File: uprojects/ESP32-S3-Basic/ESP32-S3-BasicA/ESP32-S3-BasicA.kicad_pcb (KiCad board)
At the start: 2 copper layers, 5 parts, among them U1 ESP32-S3-WROOM-1x-N8R8

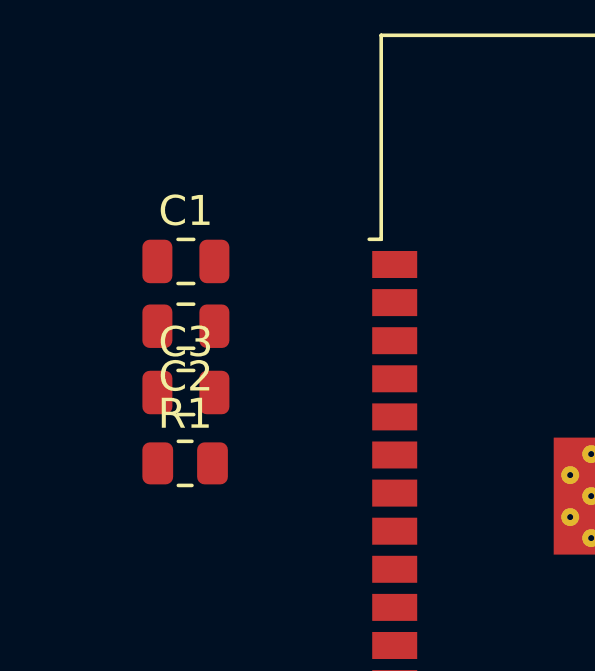
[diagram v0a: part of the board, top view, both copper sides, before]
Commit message: March 27 commit
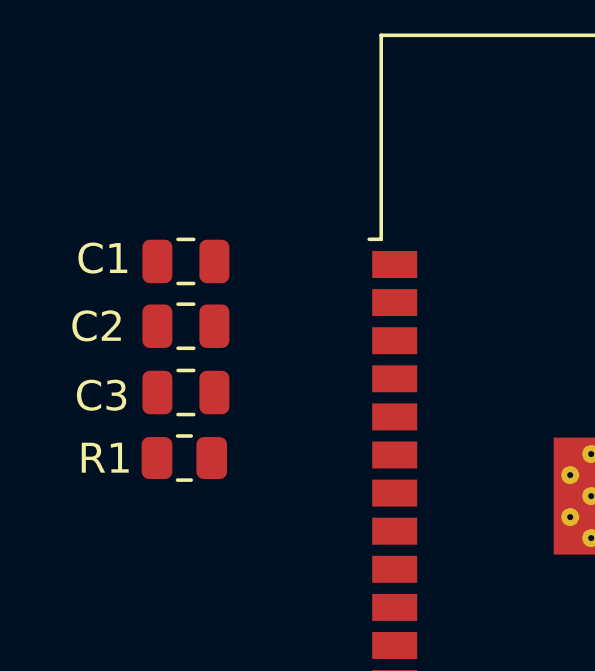
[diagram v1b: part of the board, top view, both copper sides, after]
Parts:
- moved R1 0.18 mm to (134.9, 65.5)
- turned C1 to 180 degrees
- turned C2 to 0 degrees
- turned C3 to 180 degrees
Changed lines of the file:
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@@
   (net 39 "ESP_EN")
   (footprint "Resistor_SMD:R_0805_2012Metric" (layer "F.Cu")
-    (at 134.8994 65.6336)
+    (at 134.874 65.4558)
     (descr "Resistor SMD 0805 (2012 Metric), square (rectangular) end terminal, IPC_7351 nominal, (Body size source: IPC-SM-782 page 72, https://www.pcb-3d.com/wordpress/wp-content/uploads/ipc-sm-782a_amendment_1_and_2.pdf), generated with kicad-footprint-generator")
     (tags "resistor")
@@
     (property "Sheetname" "")
     (attr smd)
-    (fp_text reference "R1" (at 0 -1.65) (layer "F.SilkS")
-        (effects (font (size 1 1) (thickness 0.15)))
-    )
-    (fp_text value "10k/R0402" (at 0 1.65) (layer "F.Fab")
+    (fp_text reference "R1" (at -2.6416 0.0254) (layer "F.SilkS")
+        (effects (font (size 1 1) (thickness 0.15)))
+    )
+    (fp_text value "10k/R0402" (at -7.8994 -8.255) (layer "F.Fab")
         (effects (font (size 1 1) (thickness 0.15)))
     )
@@
   )
   (footprint "Capacitor_SMD:C_0805_2012Metric" (layer "F.Cu")
-    (at 134.9248 61.0616 180)
+    (at 134.9248 61.0616)
     (descr "Capacitor SMD 0805 (2012 Metric), square (rectangular) end terminal, IPC_7351 nominal, (Body size source: IPC-SM-782 page 76, https://www.pcb-3d.com/wordpress/wp-content/uploads/ipc-sm-782a_amendment_1_and_2.pdf, https://docs.google.com/spreadsheets/d/1BsfQQcO9C6DZCsRaXUlFlo91Tg2WpOkGARC1WS5S8t0/edit?usp=sharing), generated with kicad-footprint-generator")
     (tags "capacitor")
@@
     (property "Sheetname" "")
     (attr smd)
-    (fp_text reference "C2" (at 0 -1.68 180) (layer "F.SilkS")
-        (effects (font (size 1 1) (thickness 0.15)))
-    )
-    (fp_text value "100nF/10V/10%/X7R/C0402" (at 6.1214 2.3368 180) (layer "F.Fab")
-        (effects (font (size 1 1) (thickness 0.15)))
-    )
-    (fp_text user "${REFERENCE}" (at 0 0 180) (layer "F.Fab")
+    (fp_text reference "C2" (at -2.9464 0.0254) (layer "F.SilkS")
+        (effects (font (size 1 1) (thickness 0.15)))
+    )
+    (fp_text value "100nF/10V/10%/X7R/C0402" (at -0.889 -7.366) (layer "F.Fab")
+        (effects (font (size 1 1) (thickness 0.15)))
+    )
+    (fp_text user "${REFERENCE}" (at 0 0) (layer "F.Fab")
         (effects (font (size 0.5 0.5) (thickness 0.08)))
     )
@@
     (fp_line (start 1 0.625) (end -1 0.625)
       (stroke (width 0.1) (type solid)) (layer "F.Fab"))
-    (pad "1" smd roundrect (at -0.95 0 180) (size 1 1.45) (layers "F.Cu" "F.Paste" "F.Mask") (roundrect_rratio 0.25)
+    (pad "1" smd roundrect (at -0.95 0) (size 1 1.45) (layers "F.Cu" "F.Paste" "F.Mask") (roundrect_rratio 0.25)
       (net 38 "GND") (pintype "passive"))
-    (pad "2" smd roundrect (at 0.95 0 180) (size 1 1.45) (layers "F.Cu" "F.Paste" "F.Mask") (roundrect_rratio 0.25)
+    (pad "2" smd roundrect (at 0.95 0) (size 1 1.45) (layers "F.Cu" "F.Paste" "F.Mask") (roundrect_rratio 0.25)
       (net 37 "+3.3V") (pintype "passive"))
     (model "${KICAD6_3DMODEL_DIR}/Capacitor_SMD.3dshapes/C_0805_2012Metric.wrl"
@@
   )
   (footprint "Capacitor_SMD:C_0805_2012Metric" (layer "F.Cu")
-    (at 134.9248 63.2714)
+    (at 134.9248 63.2714 180)
     (descr "Capacitor SMD 0805 (2012 Metric), square (rectangular) end terminal, IPC_7351 nominal, (Body size source: IPC-SM-782 page 76, https://www.pcb-3d.com/wordpress/wp-content/uploads/ipc-sm-782a_amendment_1_and_2.pdf, https://docs.google.com/spreadsheets/d/1BsfQQcO9C6DZCsRaXUlFlo91Tg2WpOkGARC1WS5S8t0/edit?usp=sharing), generated with kicad-footprint-generator")
     (tags "capacitor")
@@
     (property "Sheetname" "")
     (attr smd)
-    (fp_text reference "C3" (at 0 -1.68) (layer "F.SilkS")
-        (effects (font (size 1 1) (thickness 0.15)))
-    )
-    (fp_text value "1uF/10V/10%/X5R/C0603" (at 0 1.68) (layer "F.Fab")
+    (fp_text reference "C3" (at 2.794 -0.127) (layer "F.SilkS")
+        (effects (font (size 1 1) (thickness 0.15)))
+    )
+    (fp_text value "1uF/10V/10%/X5R/C0603" (at 1.8034 7.8486) (layer "F.Fab")
         (effects (font (size 1 1) (thickness 0.15)))
     )
@@
     (fp_line (start 1 0.625) (end -1 0.625)
       (stroke (width 0.1) (type solid)) (layer "F.Fab"))
-    (pad "1" smd roundrect (at -0.95 0) (size 1 1.45) (layers "F.Cu" "F.Paste" "F.Mask") (roundrect_rratio 0.25)
+    (pad "1" smd roundrect (at -0.95 0 180) (size 1 1.45) (layers "F.Cu" "F.Paste" "F.Mask") (roundrect_rratio 0.25)
       (net 39 "ESP_EN") (pintype "passive"))
-    (pad "2" smd roundrect (at 0.95 0) (size 1 1.45) (layers "F.Cu" "F.Paste" "F.Mask") (roundrect_rratio 0.25)
+    (pad "2" smd roundrect (at 0.95 0 180) (size 1 1.45) (layers "F.Cu" "F.Paste" "F.Mask") (roundrect_rratio 0.25)
       (net 38 "GND") (pintype "passive"))
     (model "${KICAD6_3DMODEL_DIR}/Capacitor_SMD.3dshapes/C_0805_2012Metric.wrl"
@@
   )
   (footprint "Capacitor_SMD:C_0805_2012Metric" (layer "F.Cu")
-    (at 134.9248 58.9026)
+    (at 134.9248 58.9026 180)
     (descr "Capacitor SMD 0805 (2012 Metric), square (rectangular) end terminal, IPC_7351 nominal, (Body size source: IPC-SM-782 page 76, https://www.pcb-3d.com/wordpress/wp-content/uploads/ipc-sm-782a_amendment_1_and_2.pdf, https://docs.google.com/spreadsheets/d/1BsfQQcO9C6DZCsRaXUlFlo91Tg2WpOkGARC1WS5S8t0/edit?usp=sharing), generated with kicad-footprint-generator")
     (tags "capacitor")
@@
     (property "Sheetname" "")
     (attr smd)
-    (fp_text reference "C1" (at 0 -1.68) (layer "F.SilkS")
-        (effects (font (size 1 1) (thickness 0.15)))
-    )
-    (fp_text value "22uF/6.3V/20%/X5R/C0603" (at -4.6482 -2.4638) (layer "F.Fab")
+    (fp_text reference "C1" (at 2.7432 0.0762) (layer "F.SilkS")
+        (effects (font (size 1 1) (thickness 0.15)))
+    )
+    (fp_text value "22uF/6.3V/20%/X5R/C0603" (at 1.2954 7.2136) (layer "F.Fab")
         (effects (font (size 1 1) (thickness 0.15)))
     )
@@
     (fp_line (start 1 0.625) (end -1 0.625)
       (stroke (width 0.1) (type solid)) (layer "F.Fab"))
-    (pad "1" smd roundrect (at -0.95 0) (size 1 1.45) (layers "F.Cu" "F.Paste" "F.Mask") (roundrect_rratio 0.25)
+    (pad "1" smd roundrect (at -0.95 0 180) (size 1 1.45) (layers "F.Cu" "F.Paste" "F.Mask") (roundrect_rratio 0.25)
       (net 37 "+3.3V") (pintype "passive"))
-    (pad "2" smd roundrect (at 0.95 0) (size 1 1.45) (layers "F.Cu" "F.Paste" "F.Mask") (roundrect_rratio 0.25)
+    (pad "2" smd roundrect (at 0.95 0 180) (size 1 1.45) (layers "F.Cu" "F.Paste" "F.Mask") (roundrect_rratio 0.25)
       (net 38 "GND") (pintype "passive"))
     (model "${KICAD6_3DMODEL_DIR}/Capacitor_SMD.3dshapes/C_0805_2012Metric.wrl"
